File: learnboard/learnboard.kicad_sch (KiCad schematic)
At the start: 45 parts, among them SW1 SW_Push, SW10 SW_Push, SW11 SW_Push, SW12 SW_Push, SW13 SW_Push, SW14 SW_Push, SW15 SW_Push, SW16 SW_Push, SW17 RotaryEncoder_Switch_MP, SW2 SW_Push, SW3 SW_Push, SW4 SW_Push, SW5 SW_Push, SW6 SW_Push, SW7 SW_Push, SW8 SW_Push, SW9 SW_Push, U1 PCM5100

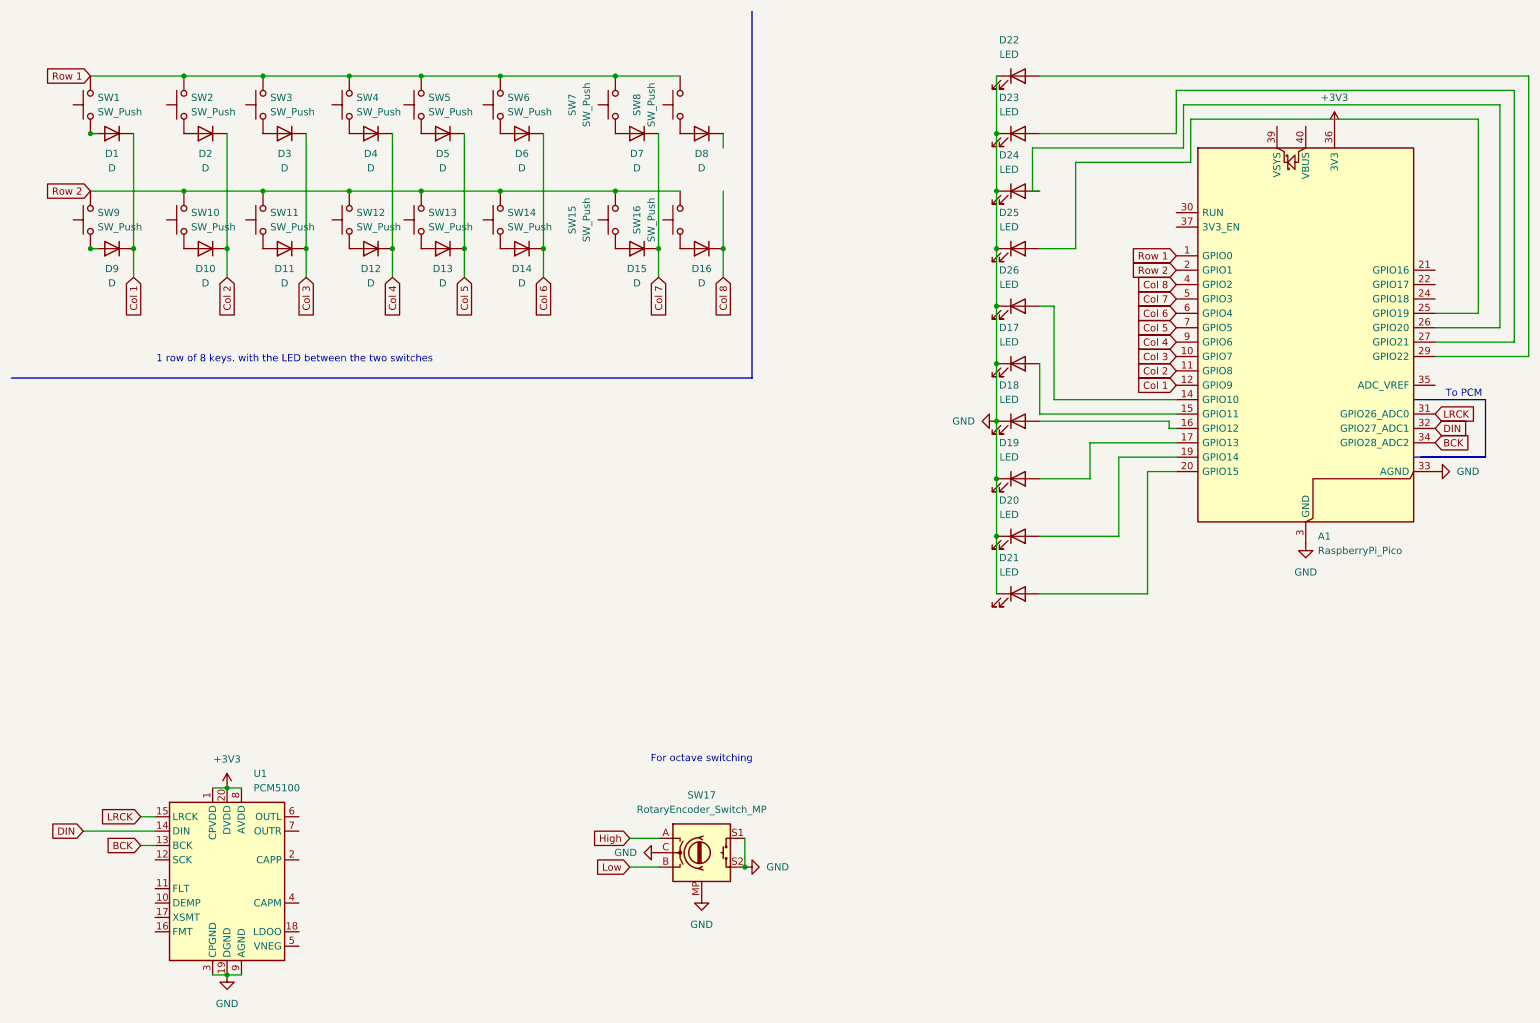
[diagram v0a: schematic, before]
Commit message: day two
worked on the pcb and fixed some things on the schematic
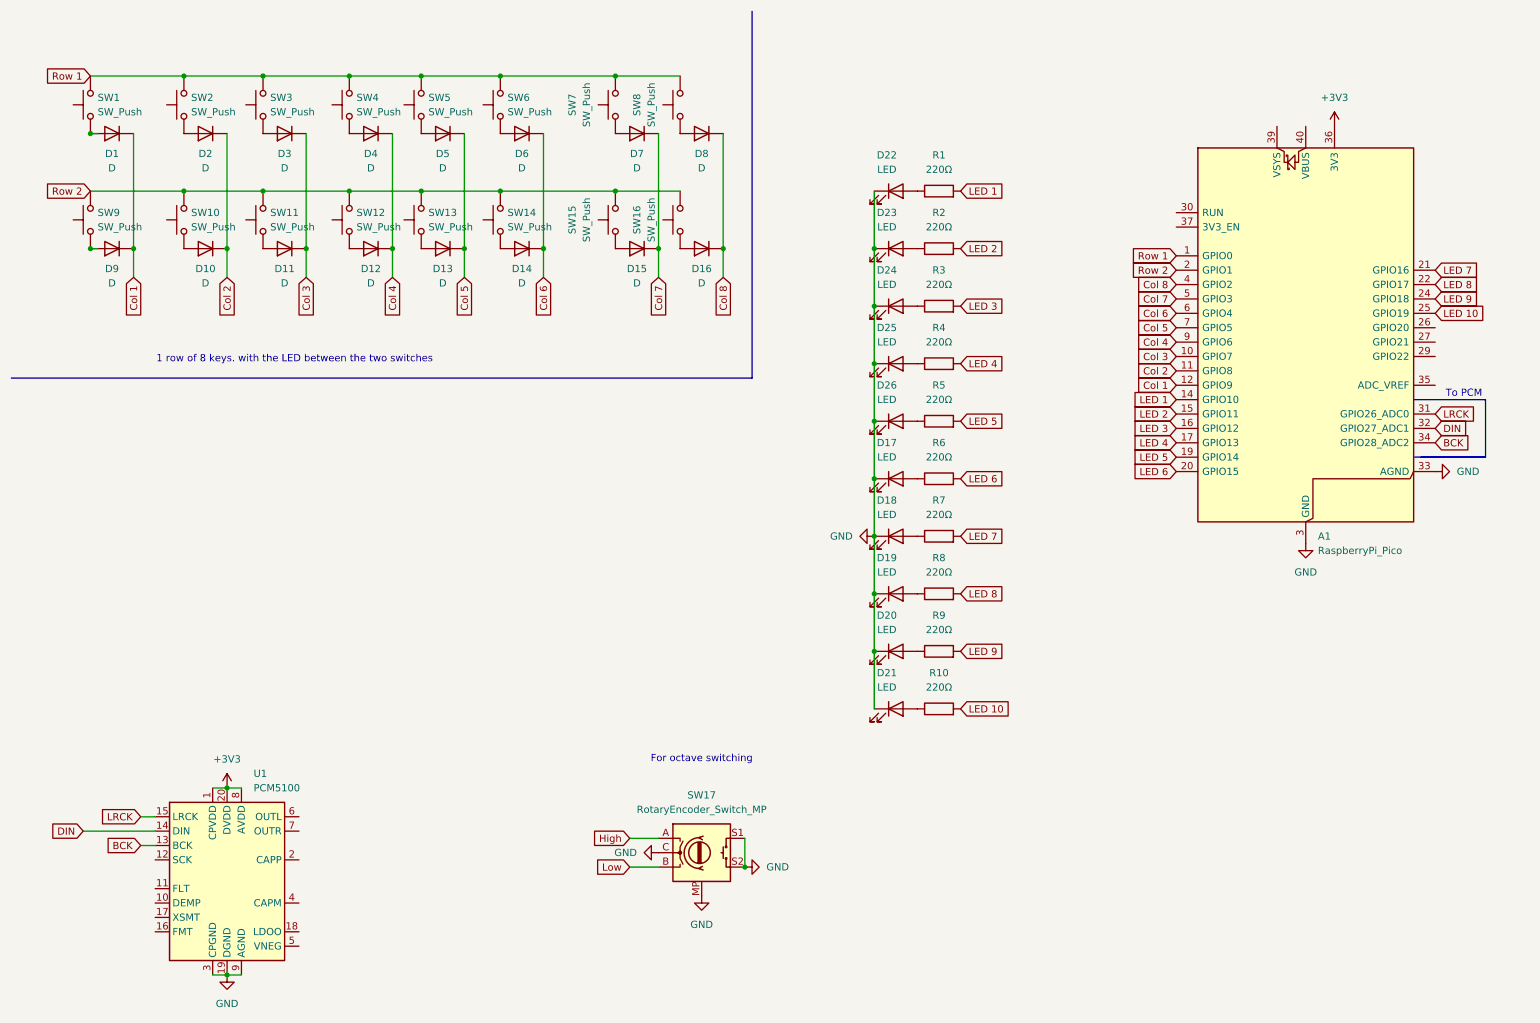
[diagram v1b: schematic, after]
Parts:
- added R1, R10, R2, R3, R4, R5, R6, R7, R8, R9: 220Ω, Resistor_THT:R_Axial_DIN0204_L3.6mm_D1.6mm_P5.08mm_Horizontal, symbol Device:R
- D1, D10, D11, D12, D13, D14, D15, D16, D2, D3, D4, D5, D6, D7, D8, D9: footprint (none) -> Diode_SMD:D_0201_0603Metric_Pad0.64x0.40mm_HandSolder
- D17, D18, D19, D20, D21, D22, D23, D24, D25, D26: footprint (none) -> LED_THT:LED_D1.8mm_W1.8mm_H2.4mm_Horizontal_O1.27mm_Z1.6mm
- SW1, SW10, SW11, SW12, SW13, SW14, SW15, SW16, SW2, SW3, SW4, SW5, SW6, SW7, SW8, SW9: footprint (none) -> Button_Switch_Keyboard:SW_Cherry_MX_1.00u_PCB
- SW17: footprint (none) -> Rotary_Encoder:RotaryEncoder_Alps_EC11E-Switch_Vertical_H20mm
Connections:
- net Col 8: now also D8.1 (K)
- net at D23.2 (A): now also R2.1; no longer A1.27 (GPIO21)
- net at D18.2 (A): now also R7.1; no longer A1.16 (GPIO12)
- net at D25.2 (A): now also R4.1; no longer A1.25 (GPIO19)
- net at D22.2 (A): now also R1.1; no longer A1.29 (GPIO22)
- net at D26.2 (A): now also R5.1; no longer A1.14 (GPIO10)
- net at D17.2 (A): now also R6.1; no longer A1.15 (GPIO11)
- net at D21.2 (A): now also R10.1; no longer A1.20 (GPIO15)
- net at D20.2 (A): now also R9.1; no longer A1.19 (GPIO14)
- net at D19.2 (A): now also R8.1; no longer A1.17 (GPIO13)
- net LED 7: now reaches A1.21 (GPIO16)
- net LED 7: now also R7.2
- net LED 8: now reaches A1.22 (GPIO17)
- net LED 8: now also R8.2
- net LED 9: now reaches A1.24 (GPIO18)
- net LED 9: now also R9.2
- net at D24.2 (A): now also R3.1; no longer A1.26 (GPIO20)
- new net LED 1: A1.14 (GPIO10), R1.2
- new net LED 10: A1.25 (GPIO19), R10.2
- new net LED 2: A1.15 (GPIO11), R2.2
- new net LED 3: A1.16 (GPIO12), R3.2
- new net LED 4: A1.17 (GPIO13), R4.2
- new net LED 5: A1.19 (GPIO14), R5.2
- new net LED 6: A1.20 (GPIO15), R6.2
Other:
- moved on the sheet: D17, D18, D19, D20, D21, D22, D23, D24, D25, D26

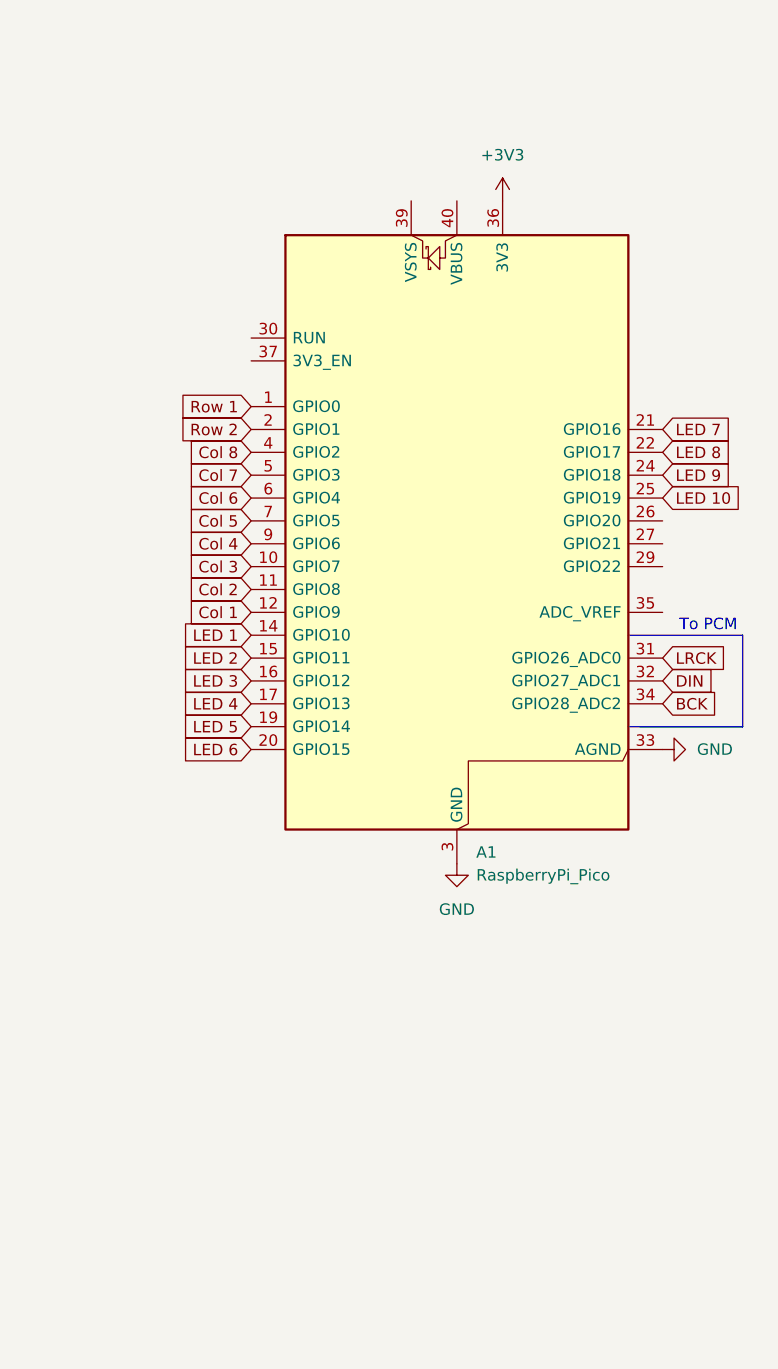
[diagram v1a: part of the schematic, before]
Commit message: tried to route things
it is not going very well.
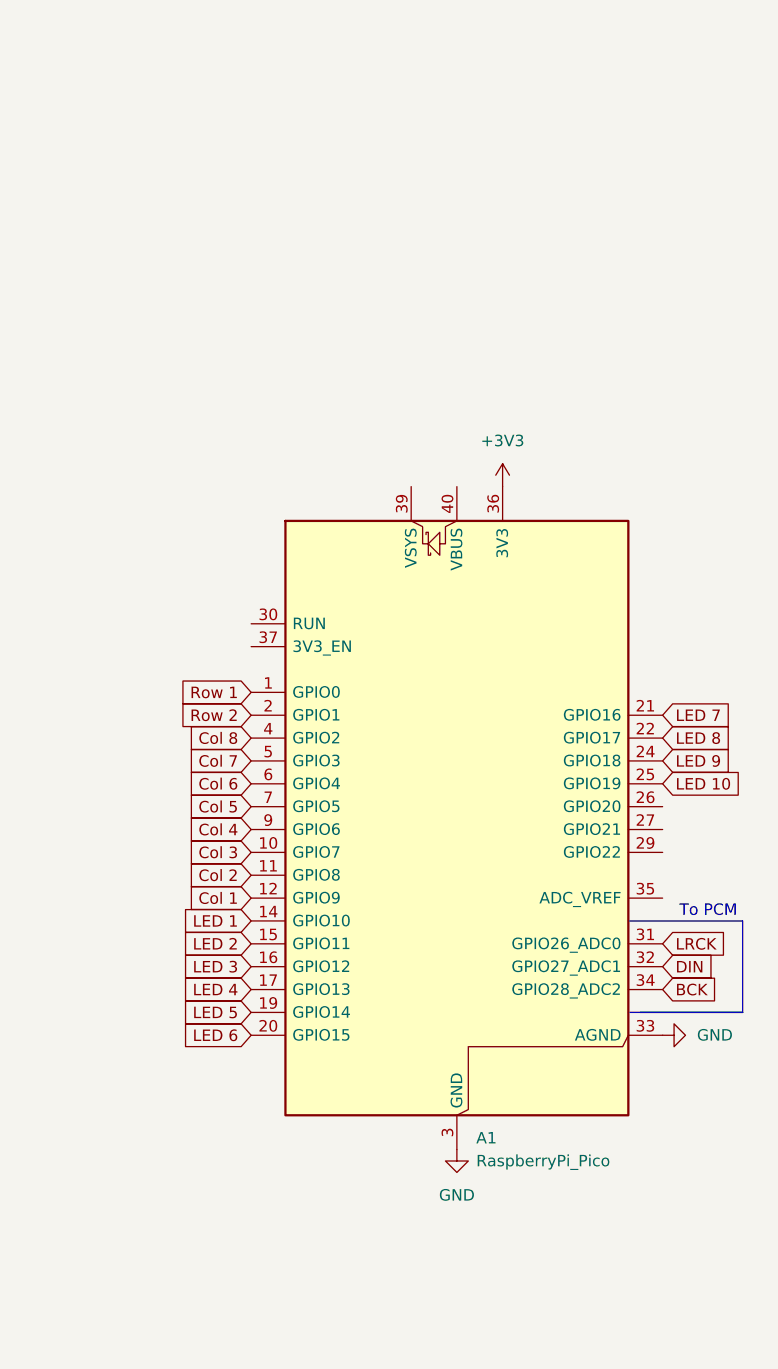
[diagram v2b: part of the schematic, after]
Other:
- moved on the sheet: A1
